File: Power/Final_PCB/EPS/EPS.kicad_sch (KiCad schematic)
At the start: 33 parts, among them J1 Left_Header, J2 Right_Header, U1 INA226, U2 MT3608-28, U3 LM2596S-5, U4 LM2596S-3.3

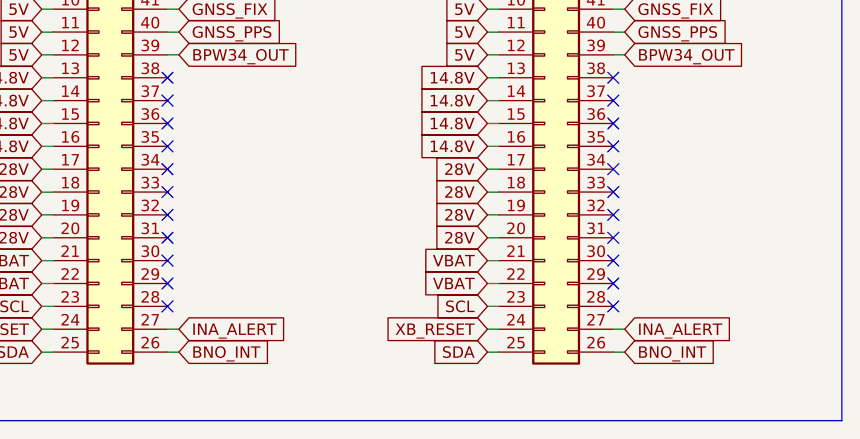
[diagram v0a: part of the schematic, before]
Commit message: Finalising Sensors Schematic
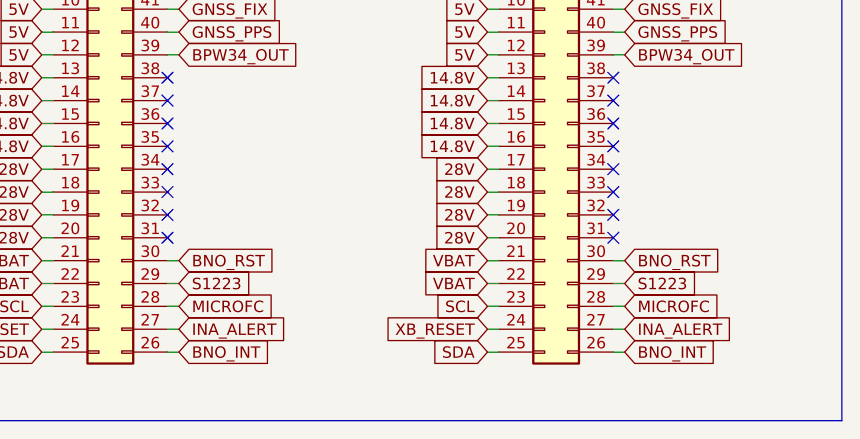
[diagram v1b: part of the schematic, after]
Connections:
- net MICROFC: now reaches J1.28 (Pin_28)
- net MICROFC: now also J2.28 (Pin_28)
- net S1223: now reaches J1.29 (Pin_29)
- net S1223: now also J2.29 (Pin_29)
- net BNO_RST: now reaches J1.30 (Pin_30)
- net BNO_RST: now also J2.30 (Pin_30)
- no-connect marks 22 -> 16
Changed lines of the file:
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@@
 	)
 	(no_connect
-		(at 259.08 95.25)
-	)
-	(no_connect
 		(at 259.08 85.09)
 	)
@@
 	)
 	(no_connect
-		(at 209.55 97.79)
-	)
-	(no_connect
 		(at 209.55 72.39)
 	)
@@
 	)
 	(no_connect
-		(at 209.55 95.25)
-	)
-	(no_connect
 		(at 259.08 74.93)
 	)
 	(no_connect
-		(at 259.08 97.79)
-	)
-	(no_connect
 		(at 209.55 90.17)
 	)
 	(no_connect
-		(at 259.08 92.71)
-	)
-	(no_connect
 		(at 259.08 90.17)
 	)
@@
 	)
 	(no_connect
-		(at 209.55 92.71)
-	)
-	(no_connect
 		(at 259.08 80.01)
 	)
@@
 	(wire
 		(pts
+			(xy 259.08 92.71) (xy 260.35 92.71)
+		)
+		(stroke
+			(width 0)
+			(type default)
+		)
+	)
+	(wire
+		(pts
 			(xy 210.82 62.23) (xy 209.55 62.23)
 		)
@@
 	(wire
 		(pts
+			(xy 209.55 95.25) (xy 210.82 95.25)
+		)
+		(stroke
+			(width 0)
+			(type default)
+		)
+	)
+	(wire
+		(pts
 			(xy 210.82 54.61) (xy 209.55 54.61)
 		)
@@
 	(wire
 		(pts
+			(xy 259.08 97.79) (xy 260.35 97.79)
+		)
+		(stroke
+			(width 0)
+			(type default)
+		)
+	)
+	(wire
+		(pts
 			(xy 162.56 34.29) (xy 162.56 35.56)
 		)
@@
 	(wire
 		(pts
+			(xy 209.55 92.71) (xy 210.82 92.71)
+		)
+		(stroke
+			(width 0)
+			(type default)
+		)
+	)
+	(wire
+		(pts
 			(xy 195.58 74.93) (xy 196.85 74.93)
 		)
@@
 	(wire
 		(pts
+			(xy 259.08 95.25) (xy 260.35 95.25)
+		)
+		(stroke
+			(width 0)
+			(type default)
+		)
+	)
+	(wire
+		(pts
 			(xy 111.76 63.5) (xy 113.03 63.5)
 		)
@@
 	(wire
 		(pts
+			(xy 209.55 97.79) (xy 210.82 97.79)
+		)
+		(stroke
+			(width 0)
+			(type default)
+		)
+	)
+	(wire
+		(pts
 			(xy 152.4 93.98) (xy 153.67 93.98)
 		)
@@
 		)
 	)
+	(global_label "MICROFC"
+		(shape input)
+		(at 260.35 97.79 0)
+		(fields_autoplaced yes)
+		(effects
+			(font
+				(size 1.27 1.27)
+			)
+			(justify left)
+		)
+		(property "Intersheetrefs" "${INTERSHEET_REFS}"
+			(at 271.6205 97.79 0)
+			(hide yes)
+			(show_name no)
+			(do_not_autoplace no)
+			(effects
+				(font
+					(size 1.27 1.27)
+				)
+				(justify left)
+			)
+		)
+	)
 	(global_label "TX2"
 		(shape input)
@@
 		)
 	)
+	(global_label "S1223"
+		(shape input)
+		(at 210.82 95.25 0)
+		(fields_autoplaced yes)
+		(effects
+			(font
+				(size 1.27 1.27)
+			)
+			(justify left)
+		)
+		(property "Intersheetrefs" "${INTERSHEET_REFS}"
+			(at 219.8527 95.25 0)
+			(hide yes)
+			(show_name no)
+			(do_not_autoplace no)
+			(effects
+				(font
+					(size 1.27 1.27)
+				)
+				(justify left)
+			)
+		)
+	)
 	(global_label "GNSS_FIX"
 		(shape input)
@@
 		)
 	)
+	(global_label "BNO_RST"
+		(shape input)
+		(at 210.82 92.71 0)
+		(fields_autoplaced yes)
+		(effects
+			(font
+				(size 1.27 1.27)
+			)
+			(justify left)
+		)
+		(property "Intersheetrefs" "${INTERSHEET_REFS}"
+			(at 222.1509 92.71 0)
+			(hide yes)
+			(show_name no)
+			(do_not_autoplace no)
+			(effects
+				(font
+					(size 1.27 1.27)
+				)
+				(justify left)
+			)
+		)
+	)
 	(global_label "VBAT"
 		(shape input)
@@
 		)
 	)
+	(global_label "MICROFC"
+		(shape input)
+		(at 210.82 97.79 0)
+		(fields_autoplaced yes)
+		(effects
+			(font
+				(size 1.27 1.27)
+			)
+			(justify left)
+		)
+		(property "Intersheetrefs" "${INTERSHEET_REFS}"
+			(at 222.0905 97.79 0)
+			(hide yes)
+			(show_name no)
+			(do_not_autoplace no)
+			(effects
+				(font
+					(size 1.27 1.27)
+				)
+				(justify left)
+			)
+		)
+	)
 	(global_label "14.8V"
 		(shape input)
@@
 		)
 	)
+	(global_label "BNO_RST"
+		(shape input)
+		(at 260.35 92.71 0)
+		(fields_autoplaced yes)
+		(effects
+			(font
+				(size 1.27 1.27)
+			)
+			(justify left)
+		)
+		(property "Intersheetrefs" "${INTERSHEET_REFS}"
+			(at 271.6809 92.71 0)
+			(hide yes)
+			(show_name no)
+			(do_not_autoplace no)
+			(effects
+				(font
+					(size 1.27 1.27)
+				)
+				(justify left)
+			)
+		)
+	)
 	(global_label "INA_14.8V"
 		(shape input)
@@
 			)
 		)
+	)
+	(global_label "S1223"
+		(shape input)
+		(at 260.35 95.25 0)
+		(fields_autoplaced yes)
+		(effects
+			(font
+				(size 1.27 1.27)
+			)
+			(justify left)
+		)
+		(property "Intersheetrefs" "${INTERSHEET_REFS}"
+			(at 269.3827 95.25 0)
+			(hide yes)
+			(show_name no)
+			(do_not_autoplace no)
+			(effects
+				(font
+					(size 1.27 1.27)
+				)
+				(justify left)
+			)
+		)

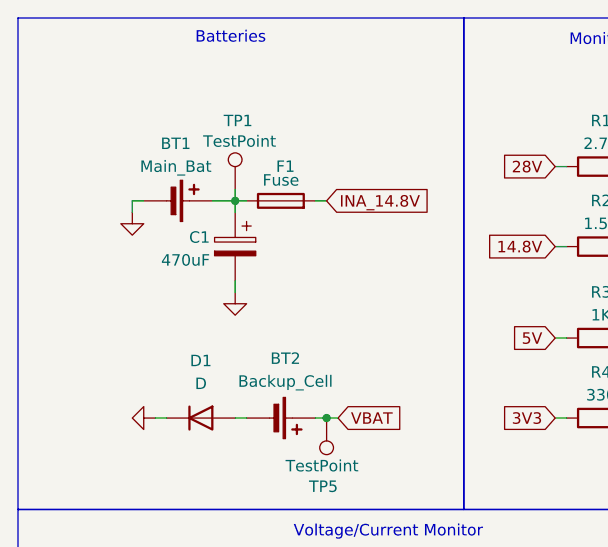
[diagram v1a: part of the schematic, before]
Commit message: Finalised Sensors PCB
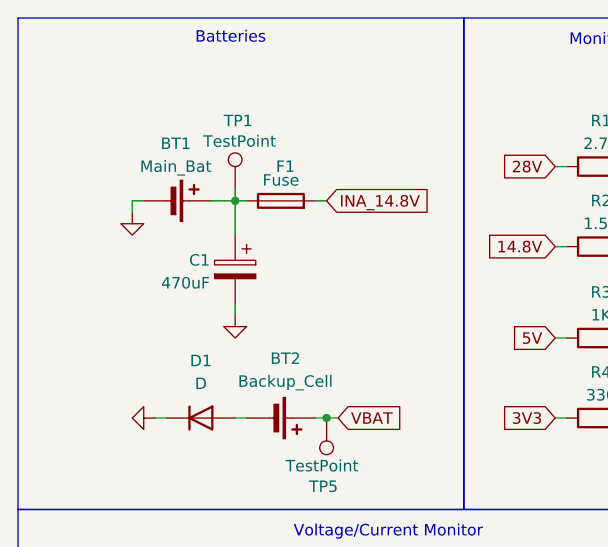
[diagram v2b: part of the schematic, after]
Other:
- moved on the sheet: C1
